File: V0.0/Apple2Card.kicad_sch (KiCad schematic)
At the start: 62 parts, among them J1 Conn_01x08_Pin, P2 Conn_02x13_Top_Bottom, SW1 SW_DIP_x08, U1C1 74LS240, U1E1 74LS14, U2 74LS133, U2B1 74LS08, U2D1 74LS138, U2E1 74LS09, U3A1 2764, U3C1 16L8, U3D1 16L8, U3E1 74LS273, U4E1 74LS245, U5A1 NCR5380, U5C1 6264, U5E1 74LS14, U6C1 74LS32, U6D1 74LS74, U6E1 74LS74

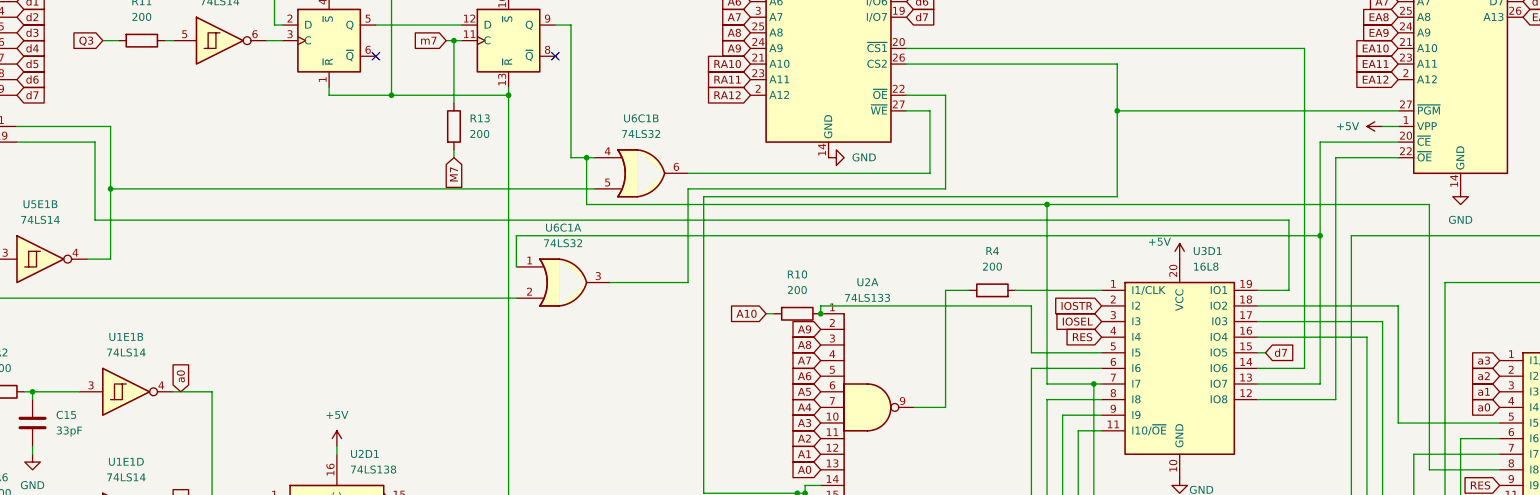
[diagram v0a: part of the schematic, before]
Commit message: menage
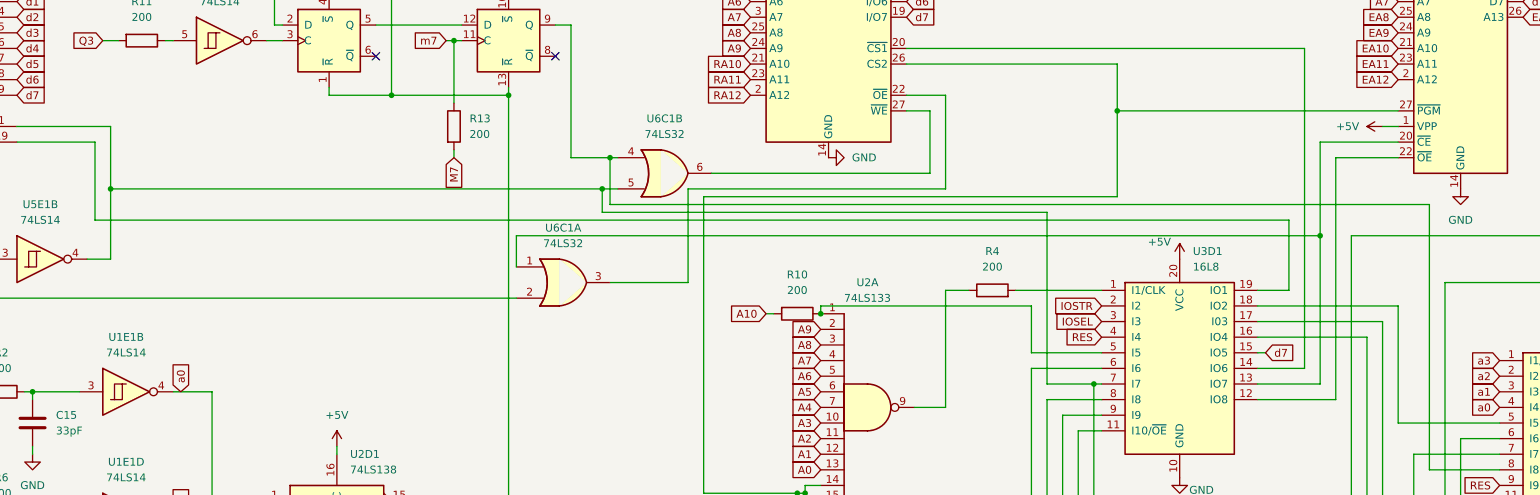
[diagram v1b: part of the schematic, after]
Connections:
- net at U4E1.1 (A->B), U5E1.4, U6C1.5: now also U3C1.7 (I7), U3D1.7 (I7)
- net at U3C1.8 (I8), U6C1.4, U6E1.9 (Q): no longer U3C1.7 (I7), U3D1.7 (I7)
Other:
- moved on the sheet: U6C1B
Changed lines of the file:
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@@
 	)
 	(junction
-		(at 393.7 143.51)
+		(at 162.56 68.58)
 		(diameter 0)
 		(color 0 0 0 0)
 	)
 	(junction
-		(at 72.39 281.94)
+		(at 393.7 143.51)
 		(diameter 0)
 		(color 0 0 0 0)
 	)
 	(junction
-		(at 137.16 49.53)
+		(at 72.39 281.94)
 		(diameter 0)
 		(color 0 0 0 0)
 	)
 	(junction
-		(at 158.75 68.58)
+		(at 137.16 49.53)
 		(diameter 0)
 		(color 0 0 0 0)
@@
 	)
 	(junction
-		(at 233.68 76.2)
-		(diameter 0)
-		(color 0 0 0 0)
-	)
-	(junction
 		(at 182.88 281.94)
 		(diameter 0)
@@
 	)
 	(junction
+		(at 161.29 73.66)
+		(diameter 0)
+		(color 0 0 0 0)
+	)
+	(junction
 		(at 311.15 147.32)
 		(diameter 0)
@@
 	(wire
 		(pts
-			(xy 175.26 71.12) (xy 214.63 71.12)
+			(xy 179.07 71.12) (xy 214.63 71.12)
 		)
 		(stroke
@@
 	(wire
 		(pts
-			(xy 156.21 68.58) (xy 158.75 68.58)
+			(xy 156.21 68.58) (xy 162.56 68.58)
 		)
 		(stroke
@@
 	(wire
 		(pts
-			(xy 158.75 68.58) (xy 158.75 76.2)
+			(xy 162.56 68.58) (xy 162.56 76.2)
 		)
 		(stroke
@@
 	(wire
 		(pts
-			(xy 81.28 73.66) (xy 160.02 73.66)
+			(xy 81.28 73.66) (xy 161.29 73.66)
 		)
 		(stroke
@@
 	(wire
 		(pts
-			(xy 158.75 68.58) (xy 160.02 68.58)
-		)
-		(stroke
-			(width 0)
-			(type default)
-		)
-	)
-	(wire
-		(pts
 			(xy 50.8 256.54) (xy 72.39 256.54)
 		)
@@
 	(wire
 		(pts
+			(xy 161.29 77.47) (xy 233.68 77.47)
+		)
+		(stroke
+			(width 0)
+			(type default)
+		)
+	)
+	(wire
+		(pts
 			(xy 91.44 106.68) (xy 97.79 106.68)
 		)
@@
 	(wire
 		(pts
+			(xy 233.68 77.47) (xy 233.68 105.41)
+		)
+		(stroke
+			(width 0)
+			(type default)
+		)
+	)
+	(wire
+		(pts
 			(xy 41.91 245.11) (xy 44.45 245.11)
 		)
@@
 	(wire
 		(pts
+			(xy 161.29 73.66) (xy 163.83 73.66)
+		)
+		(stroke
+			(width 0)
+			(type default)
+		)
+	)
+	(wire
+		(pts
 			(xy 105.41 129.54) (xy 97.79 129.54)
 		)
@@
 	(wire
 		(pts
+			(xy 161.29 73.66) (xy 161.29 77.47)
+		)
+		(stroke
+			(width 0)
+			(type default)
+		)
+	)
+	(wire
+		(pts
 			(xy 345.44 215.9) (xy 345.44 218.44)
 		)
@@
 	(wire
 		(pts
-			(xy 158.75 76.2) (xy 233.68 76.2)
-		)
-		(stroke
-			(width 0)
-			(type default)
-		)
-	)
-	(wire
-		(pts
 			(xy 307.34 116.84) (xy 293.37 116.84)
 		)
@@
 	(wire
 		(pts
-			(xy 233.68 76.2) (xy 295.91 76.2)
+			(xy 162.56 76.2) (xy 295.91 76.2)
 		)
 		(stroke
@@
 	(wire
 		(pts
-			(xy 233.68 76.2) (xy 233.68 105.41)
-		)
-		(stroke
-			(width 0)
-			(type default)
-		)
-	)
-	(wire
-		(pts
 			(xy 186.69 204.47) (xy 213.36 204.47)
 		)
@@
 	(wire
 		(pts
+			(xy 162.56 68.58) (xy 163.83 68.58)
+		)
+		(stroke
+			(width 0)
+			(type default)
+		)
+	)
+	(wire
+		(pts
 			(xy 34.29 217.17) (xy 31.75 217.17)
 		)
@@
 	(symbol
 		(lib_id "74xx:74LS32")
-		(at 167.64 71.12 0)
+		(at 171.45 71.12 0)
 		(unit 2)
 		(exclude_from_sim no)
@@
 		(fields_autoplaced yes)
 		(property "Reference" "U6C1"
-			(at 167.64 62.23 0)
+			(at 171.45 62.23 0)
 			(effects
 				(font
@@
 		)
 		(property "Value" "74LS32"
-			(at 167.64 64.77 0)
+			(at 171.45 64.77 0)
 			(effects
 				(font
@@
 		)
 		(property "Footprint" "Package_DIP:DIP-14_W7.62mm"
-			(at 167.64 71.12 0)
+			(at 171.45 71.12 0)
 			(effects
 				(font
@@
 		)
 		(property "Datasheet" "http://www.ti.com/lit/gpn/sn74LS32"
-			(at 167.64 71.12 0)
+			(at 171.45 71.12 0)
 			(effects
 				(font
@@
 		)
 		(property "Description" "Quad 2-input OR"
-			(at 167.64 71.12 0)
+			(at 171.45 71.12 0)
 			(effects
 				(font
